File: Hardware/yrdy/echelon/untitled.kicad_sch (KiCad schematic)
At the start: 3 parts, among them U2 ATxmega384D3-A, U3 BM78SPPS5NC2, U4 ESP8266EX

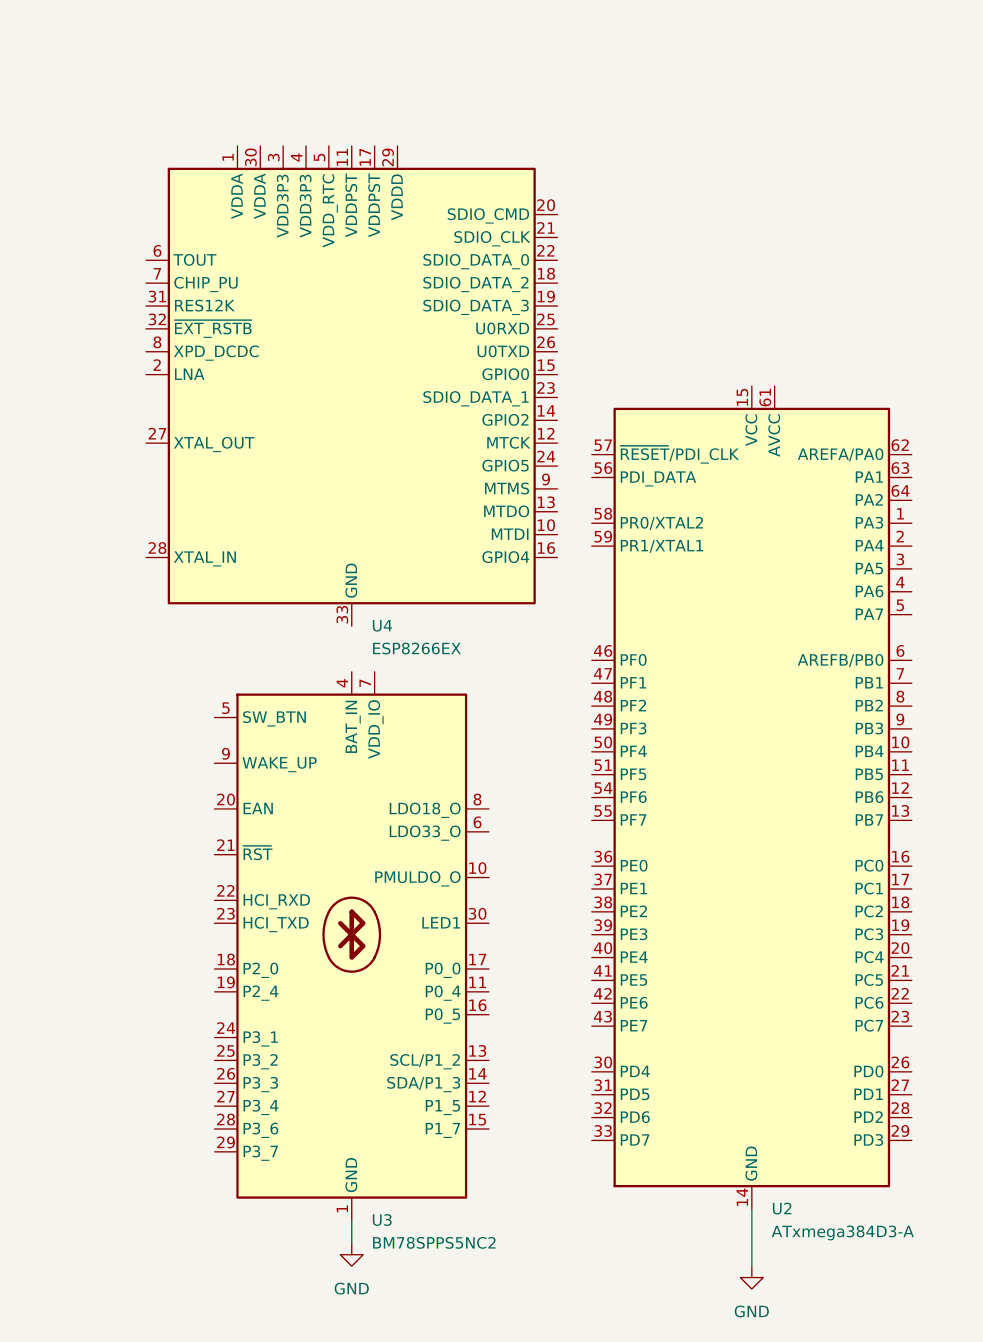
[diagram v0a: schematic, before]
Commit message: g
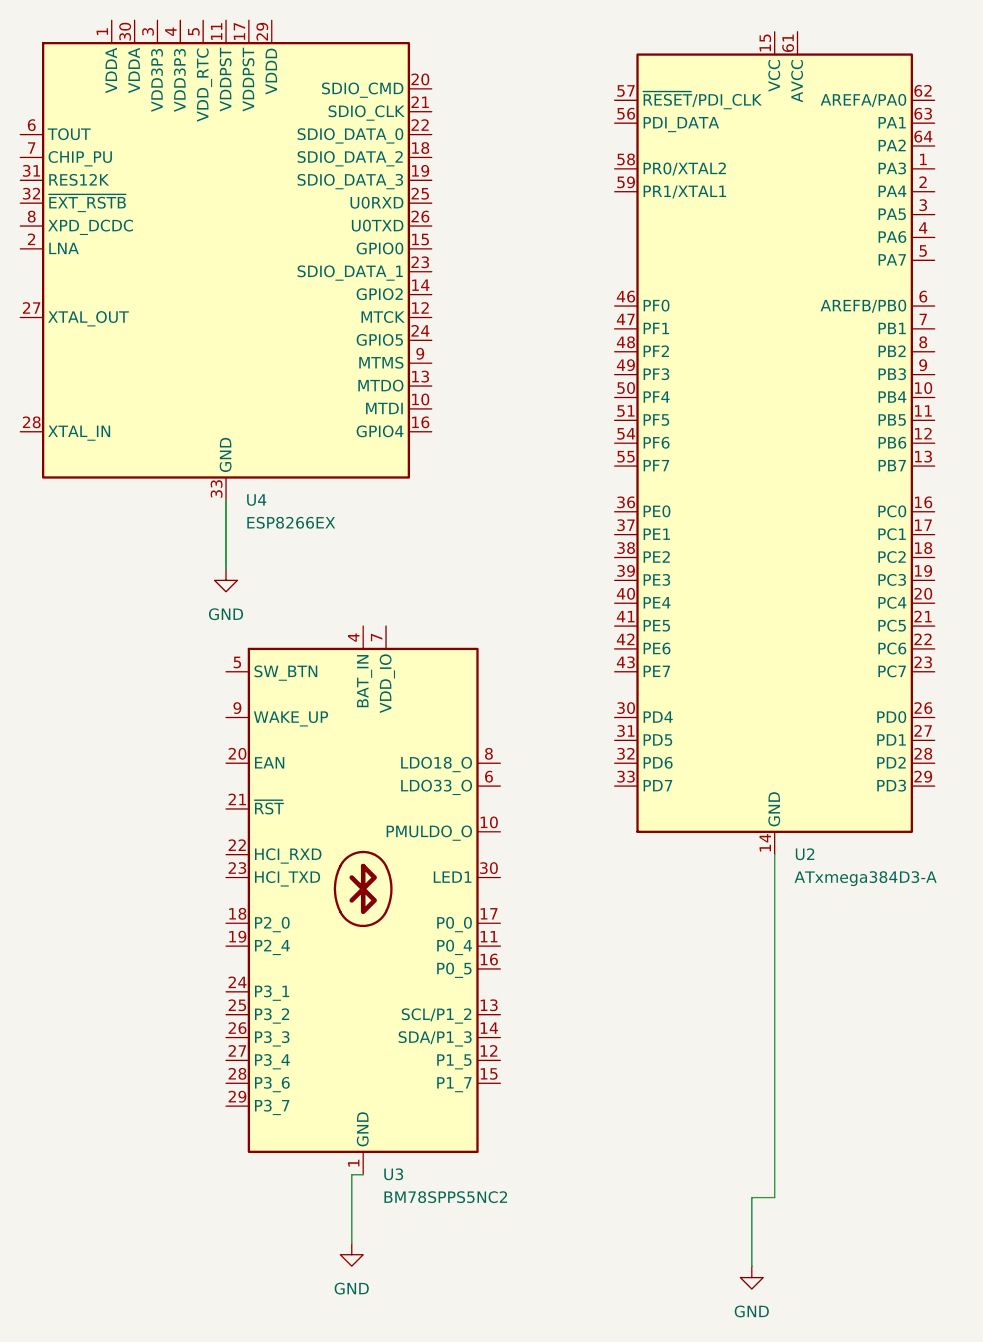
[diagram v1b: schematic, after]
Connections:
- net GND: now also U4.33 (GND)
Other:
- moved on the sheet: U2, U3, U4
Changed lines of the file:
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@@
 (kicad_sch (version 20230121) (generator eeschema)
   (paper "A4")
-  (wire (pts (xy 213.36 157.48) (xy 213.36 160.02))
-    (stroke (width 0) (type default))
-  )
-  (wire (pts (xy 257.81 156.21) (xy 257.81 162.56))
-    (stroke (width 0) (type default))
-  )
-  (symbol (lib_id "MCU_Espressif:ESP8266EX") (at 213.36 63.5 0) (unit 1)
-    (in_bom yes) (on_board yes) (dnp no) (fields_autoplaced)
-    (property "Reference" "U4" (at 215.5541 91.44 0)
-      (effects (font (size 1.27 1.27)) (justify left))
-    )
-    (property "Value" "ESP8266EX" (at 215.5541 93.98 0)
-      (effects (font (size 1.27 1.27)) (justify left))
-    )
-    (property "Footprint" "Package_DFN_QFN:QFN-32-1EP_5x5mm_P0.5mm_EP3.45x3.45mm" (at 213.36 96.52 0)
-      (effects (font (size 1.27 1.27)) hide)
-    )
-    (property "Datasheet" "http://espressif.com/sites/default/files/documentation/0a-esp8266ex_datasheet_en.pdf" (at 215.9 96.52 0)
+  (wire (pts (xy 213.36 152.4) (xy 213.36 160.02))
+    (stroke (width 0) (type default))
+  )
+  (wire (pts (xy 260.35 154.94) (xy 257.81 154.94))
+    (stroke (width 0) (type default))
+  )
+  (wire (pts (xy 260.35 116.84) (xy 260.35 154.94))
+    (stroke (width 0) (type default))
+  )
+  (wire (pts (xy 199.39 77.47) (xy 199.39 85.09))
+    (stroke (width 0) (type default))
+  )
+  (wire (pts (xy 257.81 154.94) (xy 257.81 162.56))
+    (stroke (width 0) (type default))
+  )
+  (wire (pts (xy 214.63 152.4) (xy 213.36 152.4))
+    (stroke (width 0) (type default))
+  )
+  (symbol (lib_id "MCU_Espressif:ESP8266EX") (at 199.39 49.53 0) (unit 1)
+    (in_bom yes) (on_board yes) (dnp no) (fields_autoplaced)
+    (property "Reference" "U4" (at 201.5841 77.47 0)
+      (effects (font (size 1.27 1.27)) (justify left))
+    )
+    (property "Value" "ESP8266EX" (at 201.5841 80.01 0)
+      (effects (font (size 1.27 1.27)) (justify left))
+    )
+    (property "Footprint" "Package_DFN_QFN:QFN-32-1EP_5x5mm_P0.5mm_EP3.45x3.45mm" (at 199.39 82.55 0)
+      (effects (font (size 1.27 1.27)) hide)
+    )
+    (property "Datasheet" "http://espressif.com/sites/default/files/documentation/0a-esp8266ex_datasheet_en.pdf" (at 201.93 82.55 0)
       (effects (font (size 1.27 1.27)) hide)
     )
@@
     )
   )
-  (symbol (lib_id "RF_Bluetooth:BM78SPPS5NC2") (at 213.36 127 0) (unit 1)
-    (in_bom yes) (on_board yes) (dnp no) (fields_autoplaced)
-    (property "Reference" "U3" (at 215.5541 157.48 0)
-      (effects (font (size 1.27 1.27)) (justify left))
-    )
-    (property "Value" "BM78SPPS5NC2" (at 215.5541 160.02 0)
-      (effects (font (size 1.27 1.27)) (justify left))
-    )
-    (property "Footprint" "RF_Module:BM78SPPS5XC2" (at 229.87 97.79 0)
-      (effects (font (size 1.27 1.27)) hide)
-    )
-    (property "Datasheet" "http://ww1.microchip.com/downloads/en/DeviceDoc/60001380C.pdf" (at 213.36 127 0)
+  (symbol (lib_id "RF_Bluetooth:BM78SPPS5NC2") (at 214.63 121.92 0) (unit 1)
+    (in_bom yes) (on_board yes) (dnp no) (fields_autoplaced)
+    (property "Reference" "U3" (at 216.8241 152.4 0)
+      (effects (font (size 1.27 1.27)) (justify left))
+    )
+    (property "Value" "BM78SPPS5NC2" (at 216.8241 154.94 0)
+      (effects (font (size 1.27 1.27)) (justify left))
+    )
+    (property "Footprint" "RF_Module:BM78SPPS5XC2" (at 231.14 92.71 0)
+      (effects (font (size 1.27 1.27)) hide)
+    )
+    (property "Datasheet" "http://ww1.microchip.com/downloads/en/DeviceDoc/60001380C.pdf" (at 214.63 121.92 0)
       (effects (font (size 1.27 1.27)) hide)
     )
@@
     )
   )
-  (symbol (lib_id "MCU_Microchip_ATmega:ATxmega384D3-A") (at 257.81 110.49 0) (unit 1)
-    (in_bom yes) (on_board yes) (dnp no) (fields_autoplaced)
-    (property "Reference" "U2" (at 260.0041 156.21 0)
-      (effects (font (size 1.27 1.27)) (justify left))
-    )
-    (property "Value" "ATxmega384D3-A" (at 260.0041 158.75 0)
-      (effects (font (size 1.27 1.27)) (justify left))
-    )
-    (property "Footprint" "Package_QFP:TQFP-64_14x14mm_P0.8mm" (at 257.81 110.49 0)
+  (symbol (lib_id "MCU_Microchip_ATmega:ATxmega384D3-A") (at 260.35 71.12 0) (unit 1)
+    (in_bom yes) (on_board yes) (dnp no) (fields_autoplaced)
+    (property "Reference" "U2" (at 262.5441 116.84 0)
+      (effects (font (size 1.27 1.27)) (justify left))
+    )
+    (property "Value" "ATxmega384D3-A" (at 262.5441 119.38 0)
+      (effects (font (size 1.27 1.27)) (justify left))
+    )
+    (property "Footprint" "Package_QFP:TQFP-64_14x14mm_P0.8mm" (at 260.35 71.12 0)
       (effects (font (size 1.27 1.27) italic) hide)
     )
-    (property "Datasheet" "http://ww1.microchip.com/downloads/en/DeviceDoc/Atmel-8134-8-16-bit-Atmel-XMEGA-D3-Microcontroller_Datasheet.pdf" (at 257.81 110.49 0)
+    (property "Datasheet" "http://ww1.microchip.com/downloads/en/DeviceDoc/Atmel-8134-8-16-bit-Atmel-XMEGA-D3-Microcontroller_Datasheet.pdf" (at 260.35 71.12 0)
       (effects (font (size 1.27 1.27)) hide)
     )
@@
         )
       )
+    )
+  )
+  (symbol (lib_id "power:GND") (at 199.39 85.09 0) (unit 1)
+    (in_bom yes) (on_board yes) (dnp no) (fields_autoplaced)
+    (property "Reference" "#PWR09" (at 199.39 91.44 0)
+      (effects (font (size 1.27 1.27)) hide)
+    )
+    (property "Value" "GND" (at 199.39 90.17 0)
+      (effects (font (size 1.27 1.27)))
+    )
+    (property "Footprint" "" (at 199.39 85.09 0)
+      (effects (font (size 1.27 1.27)) hide)
+    )
+    (property "Datasheet" "" (at 199.39 85.09 0)
+      (effects (font (size 1.27 1.27)) hide)
+    )
+    (pin "1")
+    (instances
+      (project "echelon"
+        (path "/5fc31bad-36d8-475d-8be1-c35c301b8728/6aedfbca-31f5-43a7-bf9d-2ecc96db9bbb"
+          (reference "#PWR09") (unit 1)
+        )
+      )
